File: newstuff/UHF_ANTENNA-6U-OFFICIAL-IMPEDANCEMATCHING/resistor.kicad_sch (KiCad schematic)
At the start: 6 parts, among them J5 Conn_01x02, J6 Conn_01x02, Q1 IRLML2052

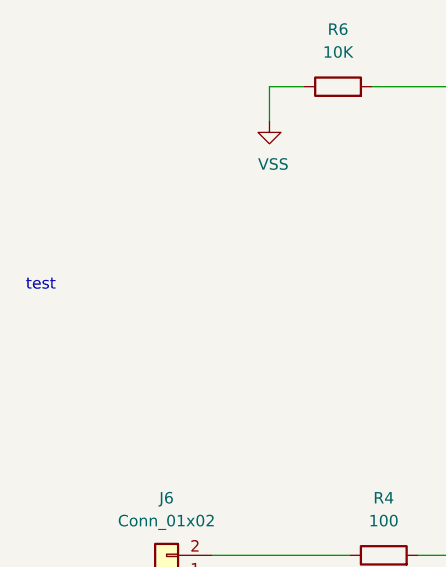
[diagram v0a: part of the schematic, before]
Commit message: fix routing
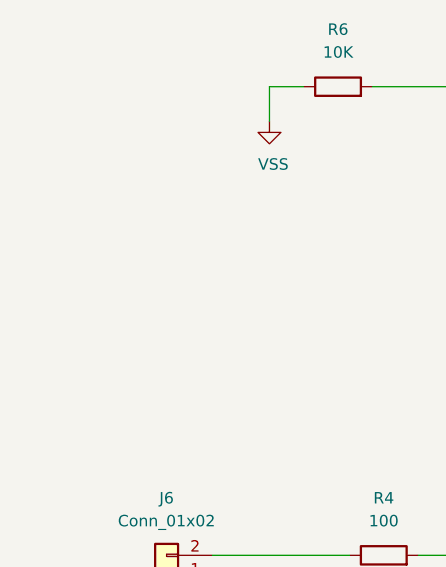
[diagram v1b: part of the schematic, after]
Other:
- note removed: "test"
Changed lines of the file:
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@@
-		)
-	)
-	(text "test"
-		(exclude_from_sim no)
-		(at 96.52 93.218 0)
-		(effects
-			(font
-				(size 1.27 1.27)
-			)
 		)
 	)

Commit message: Update resistor.kicad_sch
test
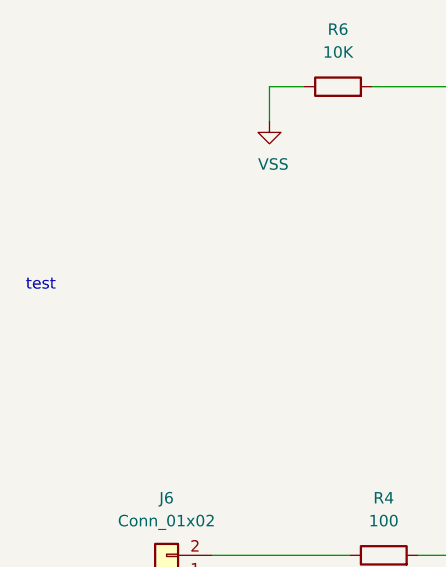
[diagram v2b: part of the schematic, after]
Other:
- note added: "test"
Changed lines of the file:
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@@
+		)
+	)
+	(text "test"
+		(exclude_from_sim no)
+		(at 96.52 93.218 0)
+		(effects
+			(font
+				(size 1.27 1.27)
+			)
 		)
 	)
